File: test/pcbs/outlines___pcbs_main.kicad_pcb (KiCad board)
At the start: 2 copper layers, 38 x 19 mm, 0 parts

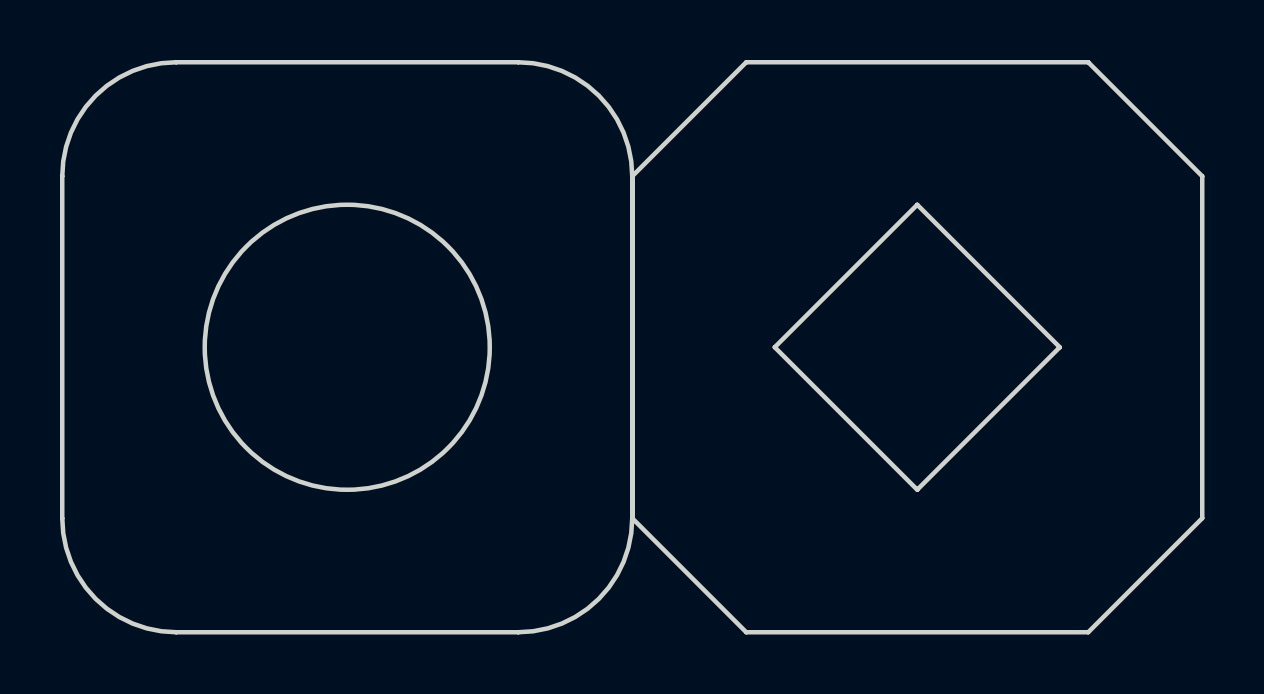
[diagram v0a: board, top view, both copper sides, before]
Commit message: ✅ Fix tests
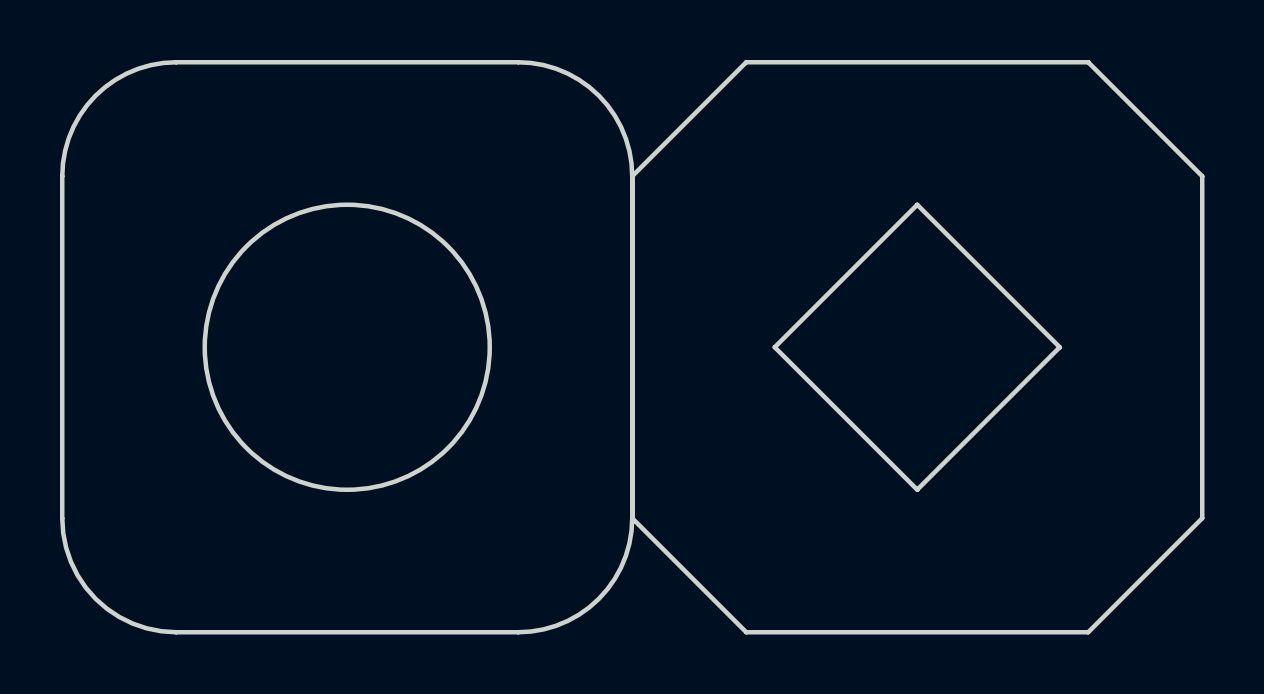
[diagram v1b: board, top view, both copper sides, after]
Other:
- net class Power added: clearance 0.2, trace_width 0.5, via_dia 0.8, via_drill 0.4
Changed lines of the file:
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@@
-(kicad_pcb (version 20171130) (host pcbnew 5.1.6)
-  (page A3)
+(kicad_pcb (version 20211014) (generator pcbnew)
+  (paper "A3")
   (title_block
-    (title main)
-    (rev v1.0.0)
-    (company Unknown)
+    (title "main")
+    (rev "v1.0.0")
+    (company "Unknown")
   )
   (general
@@
   )
   (layers
-    (0 F.Cu signal)
-    (31 B.Cu signal)
-    (32 B.Adhes user)
-    (33 F.Adhes user)
-    (34 B.Paste user)
-    (35 F.Paste user)
-    (36 B.SilkS user)
-    (37 F.SilkS user)
-    (38 B.Mask user)
-    (39 F.Mask user)
-    (40 Dwgs.User user)
-    (41 Cmts.User user)
-    (42 Eco1.User user)
-    (43 Eco2.User user)
-    (44 Edge.Cuts user)
-    (45 Margin user)
-    (46 B.CrtYd user)
-    (47 F.CrtYd user)
-    (48 B.Fab user)
-    (49 F.Fab user)
+    (0 "F.Cu" signal)
+    (31 "B.Cu" signal)
+    (32 "B.Adhes" user "B.Adhesive")
+    (33 "F.Adhes" user "F.Adhesive")
+    (34 "B.Paste" user)
+    (35 "F.Paste" user)
+    (36 "B.SilkS" user "B.Silkscreen")
+    (37 "F.SilkS" user "F.Silkscreen")
+    (38 "B.Mask" user)
+    (39 "F.Mask" user)
+    (40 "Dwgs.User" user "User.Drawings")
+    (41 "Cmts.User" user "User.Comments")
+    (42 "Eco1.User" user "User.Eco1")
+    (43 "Eco2.User" user "User.Eco2")
+    (44 "Edge.Cuts" user)
+    (45 "Margin" user)
+    (46 "B.CrtYd" user "B.Courtyard")
+    (47 "F.CrtYd" user "F.Courtyard")
+    (48 "B.Fab" user)
+    (49 "F.Fab" user)
   )
   (setup
@@
     (add_net "")
   )
-            (gr_line (start -5.7 9.5) (end 5.699999999999999 9.5) (angle 90) (layer Edge.Cuts) (width 0.15))
-(gr_line (start 9.5 5.7) (end 9.5 -5.699999999999999) (angle 90) (layer Edge.Cuts) (width 0.15))
-(gr_line (start 5.699999999999999 -9.5) (end -5.7 -9.5) (angle 90) (layer Edge.Cuts) (width 0.15))
-(gr_line (start -9.5 -5.699999999999999) (end -9.5 5.7) (angle 90) (layer Edge.Cuts) (width 0.15))
-(gr_arc (start 5.7 5.7) (end 5.7 9.5) (angle -90) (layer Edge.Cuts) (width 0.15))
-(gr_arc (start 5.7 -5.7) (end 9.5 -5.7) (angle -90) (layer Edge.Cuts) (width 0.15))
-(gr_arc (start -5.7 -5.7) (end -5.7 -9.5) (angle -90) (layer Edge.Cuts) (width 0.15))
-(gr_arc (start -5.7 5.7) (end -9.5 5.7) (angle -90) (layer Edge.Cuts) (width 0.15))
-(gr_circle (center 0 0) (end 4.75 0) (layer Edge.Cuts) (width 0.15))
-(gr_line (start 13.3 9.5) (end 9.5 5.7) (angle 90) (layer Edge.Cuts) (width 0.15))
-(gr_line (start 9.5 5.7) (end 9.5 -5.7) (angle 90) (layer Edge.Cuts) (width 0.15))
-(gr_line (start 9.5 -5.7) (end 13.3 -9.5) (angle 90) (layer Edge.Cuts) (width 0.15))
-(gr_line (start 13.3 -9.5) (end 24.700000000000003 -9.5) (angle 90) (layer Edge.Cuts) (width 0.15))
-(gr_line (start 24.700000000000003 -9.5) (end 28.5 -5.7) (angle 90) (layer Edge.Cuts) (width 0.15))
-(gr_line (start 28.5 -5.7) (end 28.5 5.7) (angle 90) (layer Edge.Cuts) (width 0.15))
-(gr_line (start 28.5 5.7) (end 24.700000000000003 9.5) (angle 90) (layer Edge.Cuts) (width 0.15))
-(gr_line (start 24.700000000000003 9.5) (end 13.3 9.5) (angle 90) (layer Edge.Cuts) (width 0.15))
-(gr_line (start 19 4.75) (end 14.25 0) (angle 90) (layer Edge.Cuts) (width 0.15))
-(gr_line (start 14.25 0) (end 19 -4.75) (angle 90) (layer Edge.Cuts) (width 0.15))
-(gr_line (start 19 -4.75) (end 23.75 0) (angle 90) (layer Edge.Cuts) (width 0.15))
-(gr_line (start 23.75 0) (end 19 4.75) (angle 90) (layer Edge.Cuts) (width 0.15))
+  (net_class Power "This is the power net class."
+    (clearance 0.2)
+    (trace_width 0.5)
+    (via_dia 0.8)
+    (via_drill 0.4)
+    (uvia_dia 0.3)
+    (uvia_drill 0.1)
+  )
+            (gr_line (start -5.7 9.5) (end 5.699999999999999 9.5) (layer "Edge.Cuts") (width 0.15))
+(gr_line (start 9.5 5.7) (end 9.5 -5.699999999999999) (layer "Edge.Cuts") (width 0.15))
+(gr_line (start 5.699999999999999 -9.5) (end -5.7 -9.5) (layer "Edge.Cuts") (width 0.15))
+(gr_line (start -9.5 -5.699999999999999) (end -9.5 5.7) (layer "Edge.Cuts") (width 0.15))
+(gr_arc (start 5.699999999999999 9.5) (mid 8.38700576850888 8.387005768508882) (end 9.5 5.700000000000001) (layer "Edge.Cuts") (width 0.15))
+(gr_arc (start 9.5 -5.7) (mid 8.387005768508882 -8.38700576850888) (end 5.7 -9.5) (layer "Edge.Cuts") (width 0.15))
+(gr_arc (start -5.7 -9.5) (mid -8.38700576850888 -8.387005768508882) (end -9.5 -5.700000000000001) (layer "Edge.Cuts") (width 0.15))
+(gr_arc (start -9.5 5.699999999999999) (mid -8.387005768508882 8.38700576850888) (end -5.700000000000001 9.5) (layer "Edge.Cuts") (width 0.15))
+(gr_circle (center 0 0) (end 4.75 0) (layer "Edge.Cuts") (width 0.15))
+(gr_line (start 13.3 9.5) (end 9.5 5.7) (layer "Edge.Cuts") (width 0.15))
+(gr_line (start 9.5 5.7) (end 9.5 -5.7) (layer "Edge.Cuts") (width 0.15))
+(gr_line (start 9.5 -5.7) (end 13.3 -9.5) (layer "Edge.Cuts") (width 0.15))
+(gr_line (start 13.3 -9.5) (end 24.700000000000003 -9.5) (layer "Edge.Cuts") (width 0.15))
+(gr_line (start 24.700000000000003 -9.5) (end 28.5 -5.7) (layer "Edge.Cuts") (width 0.15))
+(gr_line (start 28.5 -5.7) (end 28.5 5.7) (layer "Edge.Cuts") (width 0.15))
+(gr_line (start 28.5 5.7) (end 24.700000000000003 9.5) (layer "Edge.Cuts") (width 0.15))
+(gr_line (start 24.700000000000003 9.5) (end 13.3 9.5) (layer "Edge.Cuts") (width 0.15))
+(gr_line (start 19 4.75) (end 14.25 0) (layer "Edge.Cuts") (width 0.15))
+(gr_line (start 14.25 0) (end 19 -4.75) (layer "Edge.Cuts") (width 0.15))
+(gr_line (start 19 -4.75) (end 23.75 0) (layer "Edge.Cuts") (width 0.15))
+(gr_line (start 23.75 0) (end 19 4.75) (layer "Edge.Cuts") (width 0.15))
 )
